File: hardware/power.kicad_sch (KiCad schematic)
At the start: 44 parts, among them J1 B2B-PH-K-S, J2 DX07S016JA1R1500, J3 PRPC001DAAN-RC, J4 PRPC001DAAN-RC, J5 PRPC001DAAN-RC, J6 PRPC001DAAN-RC, J7 PRPC001DAAN-RC, Q1 IRLML2246TRPBF, Q2 IRLML6344TRPBF, Q3 IRLML6344TRPBF, U1 USBLC6-2SC6, U2 S-8240ADQ-M6T1U, U3 BQ21040DBVR, U4 LM66200DRLR, U5 TPS63031DSK

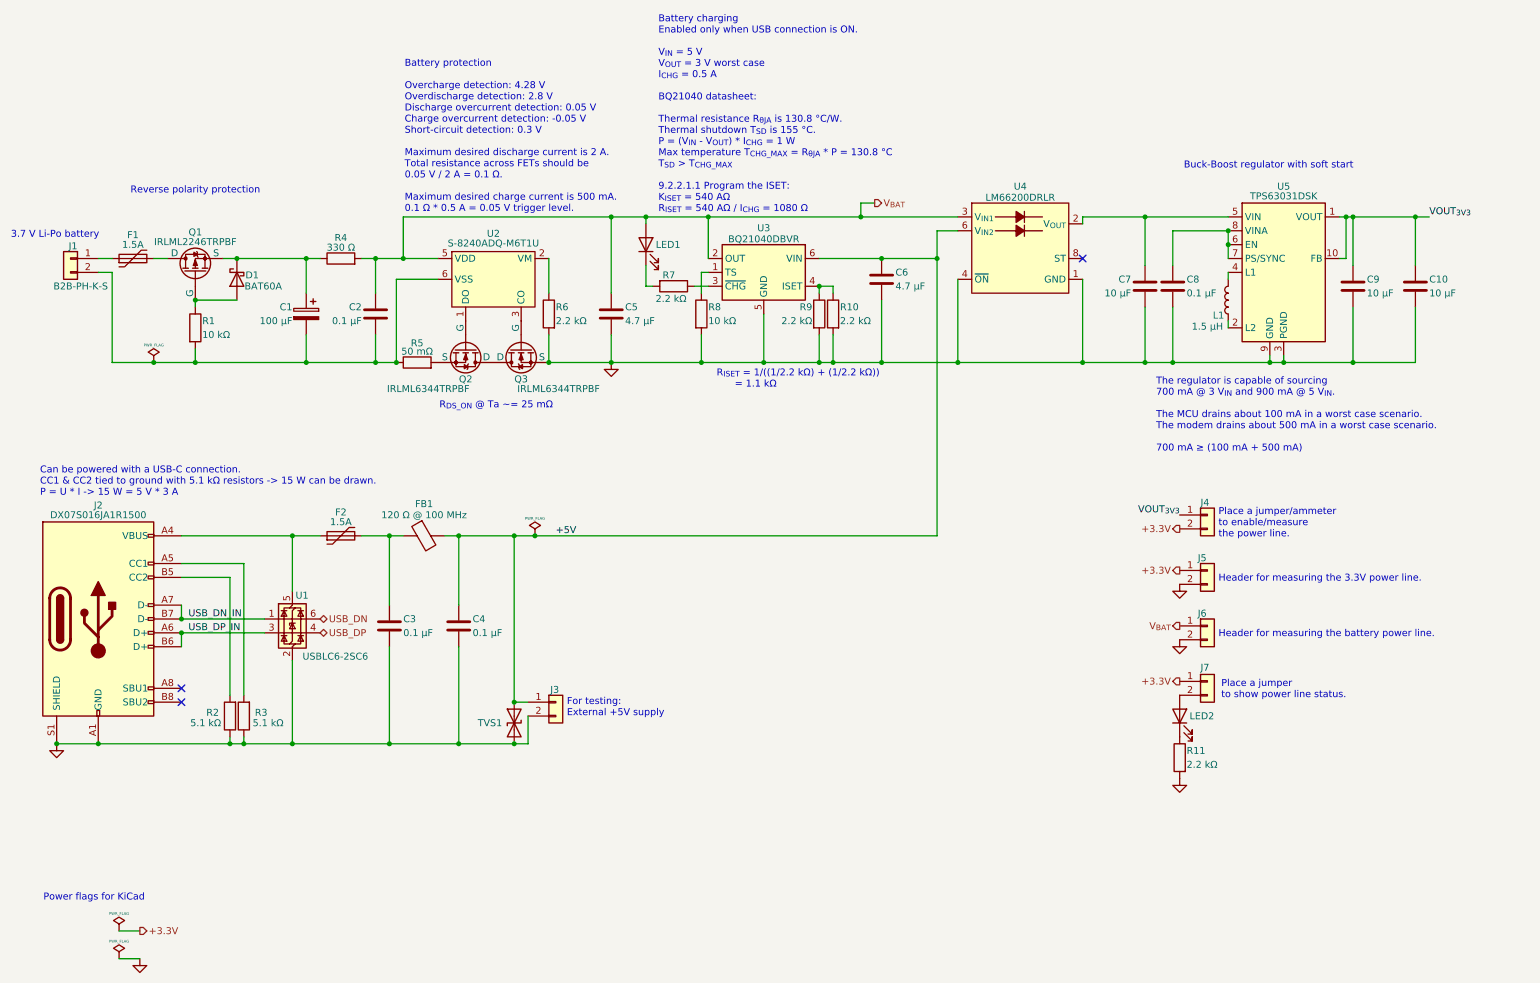
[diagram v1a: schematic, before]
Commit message: HW: Refine schematics
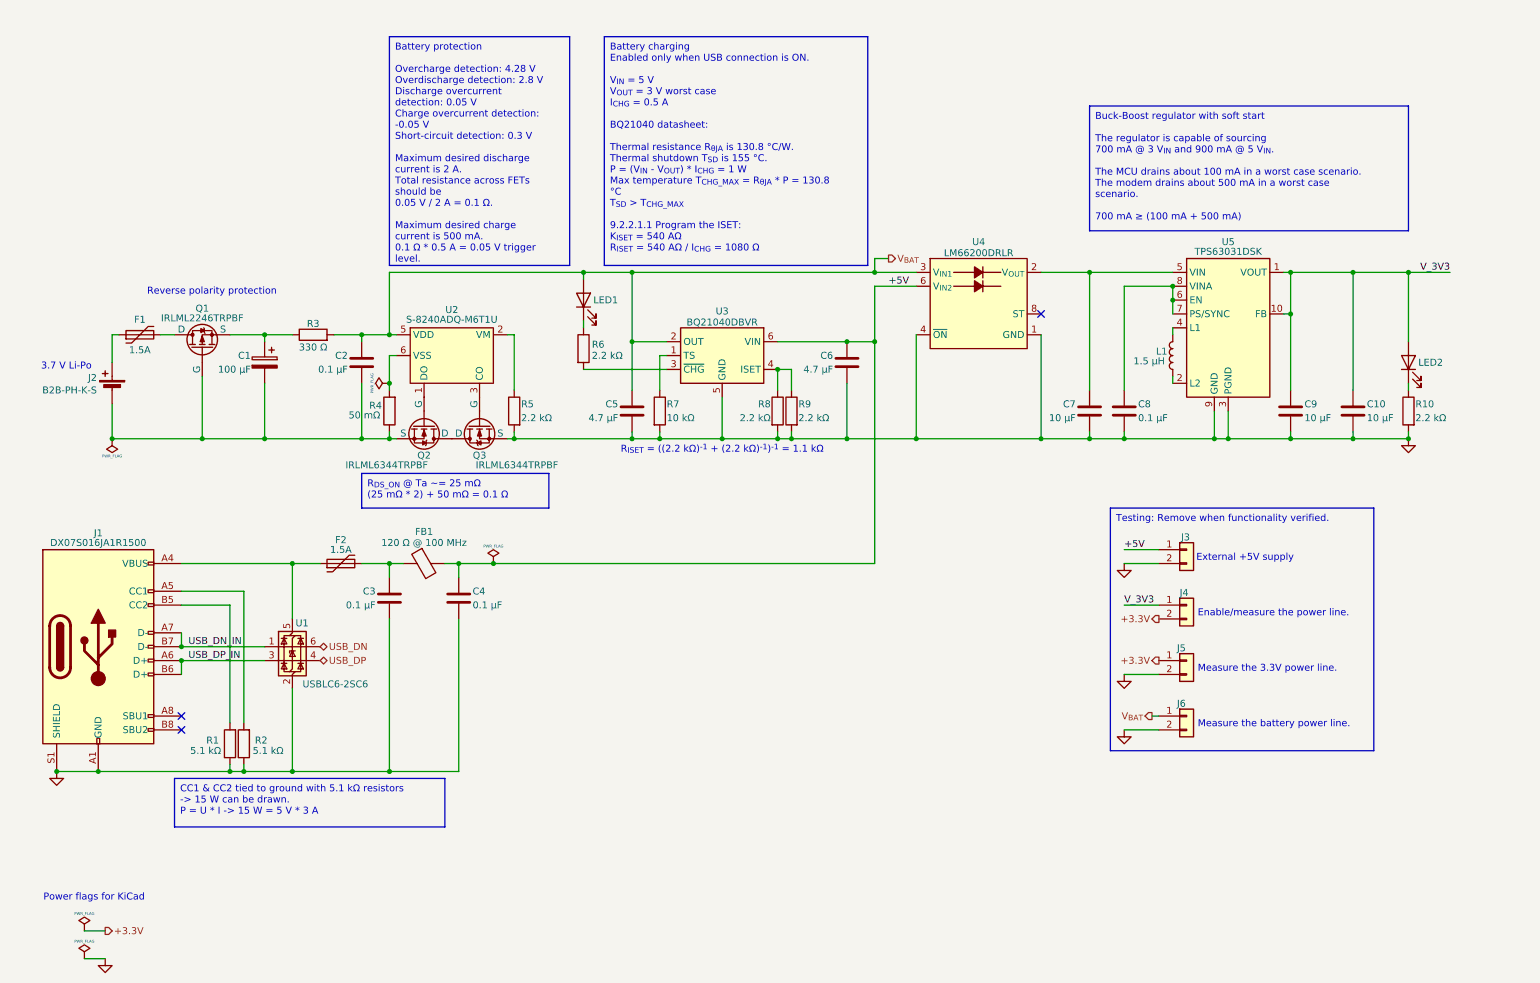
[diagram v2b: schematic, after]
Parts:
- removed D1: BAT60A, Diode_SMD:D_SOD-323_HandSoldering, symbol Device:D_Schottky
- removed J7: PRPC001DAAN-RC, Connector_PinHeader_2.54mm:PinHeader_1x02_P2.54mm_Vertical, symbol Connector_Generic:Conn_01x02
- removed R1: 10 kΩ, Resistor_SMD:R_0603_1608Metric_Pad0.98x0.95mm_HandSolder, symbol Device:R
- removed TVS1: SMAJ6.0CA, Diode_SMD:D_SMA_Handsoldering, symbol Device:D_TVS
- J2: renamed from J1; symbol Connector_Generic:Conn_01x02 -> Device:Battery_Cell
- renumbered J2 to J1, R2 to R1, R11 to R10, R3 to R2, R4 to R3, R5 to R4, R6 to R5, R7 to R6, R8 to R7, R9 to R8, R10 to R9
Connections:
- net VOUT_{3V3} is gone; now on net V_3V3: C10.1, C9.1, J4.1 (Pin_1), U5.1 (VOUT), U5.10 (FB)
- net at C1.2, C2.2, J2.2 (-)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: now also Q1.1 (G), Q2.2 (S); no longer U2.6 (VSS)
- net at R4.2: now also U2.6 (VSS); no longer Q2.2 (S)
- net V_3V3: now reaches LED2.2 (A)
- net at R6.1: now also LED1.1 (K); no longer U3.3 (~{CHG})
- net at R6.2: now also U3.3 (~{CHG}); no longer LED1.1 (K)
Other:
- note added: "3.7 V Li-Po"
- note added: "Enable/measure the power line."
- note added: "External +5V supply"
- note added: "Measure the 3.3V power line."
- note added: "Measure the battery power line."
- note added: "R_{ISET} = ((2.2 kΩ)^{-1} + (2.2 kΩ)^{-1})^{-1} = 1.1 kΩ"
- note removed: "3.7 V Li-Po battery"
- note removed: "Battery charging Enabled only when USB connection is ON. V_{IN} = 5 V V_{OUT} = 3 V worst case I_{CHG} = 0.5 A BQ21040 datasheet: Thermal resistance R_{θJA} is 130.8 °C/W. Thermal shutdown T_{SD} is 155 °C. P = (V_{IN} - V_{OUT}) * I_{CHG} = 1 W Max temperature T_{CHG_MAX} = R_{θJA} * P = 130.8 °C T_{SD} > T_{CHG_MAX} 9.2.2.1.1 Program the ISET: K_{ISET} = 540 AΩ R_{ISET} = 540 AΩ / I_{CHG} = 108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"
- note removed: "Battery protection Overcharge detection: 4.28 V Overdischarge detection: 2.8 V Discharge overcurrent detection: 0.05 V Charge overcurrent detection: -0.05 V Short-circuit detection: 0.3 V Maximum desired discharge current is 2 A. Total resistance across FETs should be 0.05 V / 2 A = 0.1 Ω. Maximum desired charge current is 500 mA. 0.1 Ω * 0.5 A = 0.05 V trigger level."
- note removed: "Buck-Boost regulator with soft start"
- note removed: "Can be powered with a USB-C connection. CC1 & CC2 tied to ground with 5.1 kΩ resistors -> 15 W can be drawn. P = U * I -> 15 W = 5 V * 3 A"
- note removed: "For testing: External +5V supply"
- note removed: "Header for measuring the 3.3V power line."
- note removed: "Header for measuring the battery power line."
- note removed: "Place a jumper to show power line status."
- note removed: "Place a jumper/ammeter to enable/measure the power line."
- note removed: "R_{DS_ON} @ Ta ~= 25 mΩ"
- note removed: "R_{ISET} = 1/((1/2.2 kΩ) + (1/2.2 kΩ)) = 1.1 kΩ"
- note removed: "The regulator is capable of sourcing 700 mA @ 3 V_{IN} and 900 mA @ 5 V_{IN}. The MCU drains about 100 mA in a worst case scenario. The modem drains about 500 mA in a worst case scenario. 700 mA ≥ (100 mA + 500 mA)"
- moved on the sheet: C1, C10, C2, C3, C4, C5, C6, C7, C8, C9, F1, F2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
